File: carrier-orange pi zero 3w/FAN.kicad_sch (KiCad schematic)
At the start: 11 parts, among them J15 FAN1, J16 FAN2, Q3 AO3400A, Q4 AO3400A

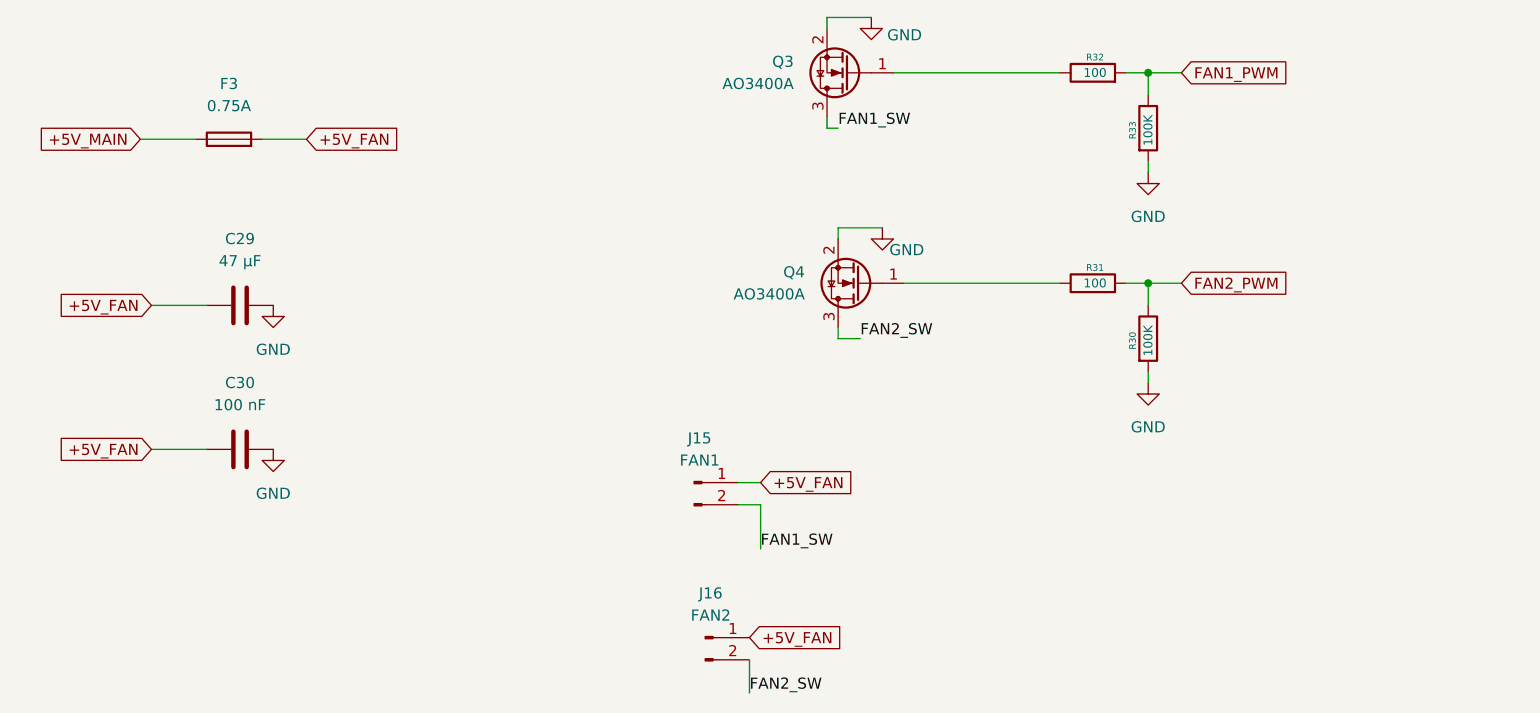
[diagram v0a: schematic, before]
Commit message: ain
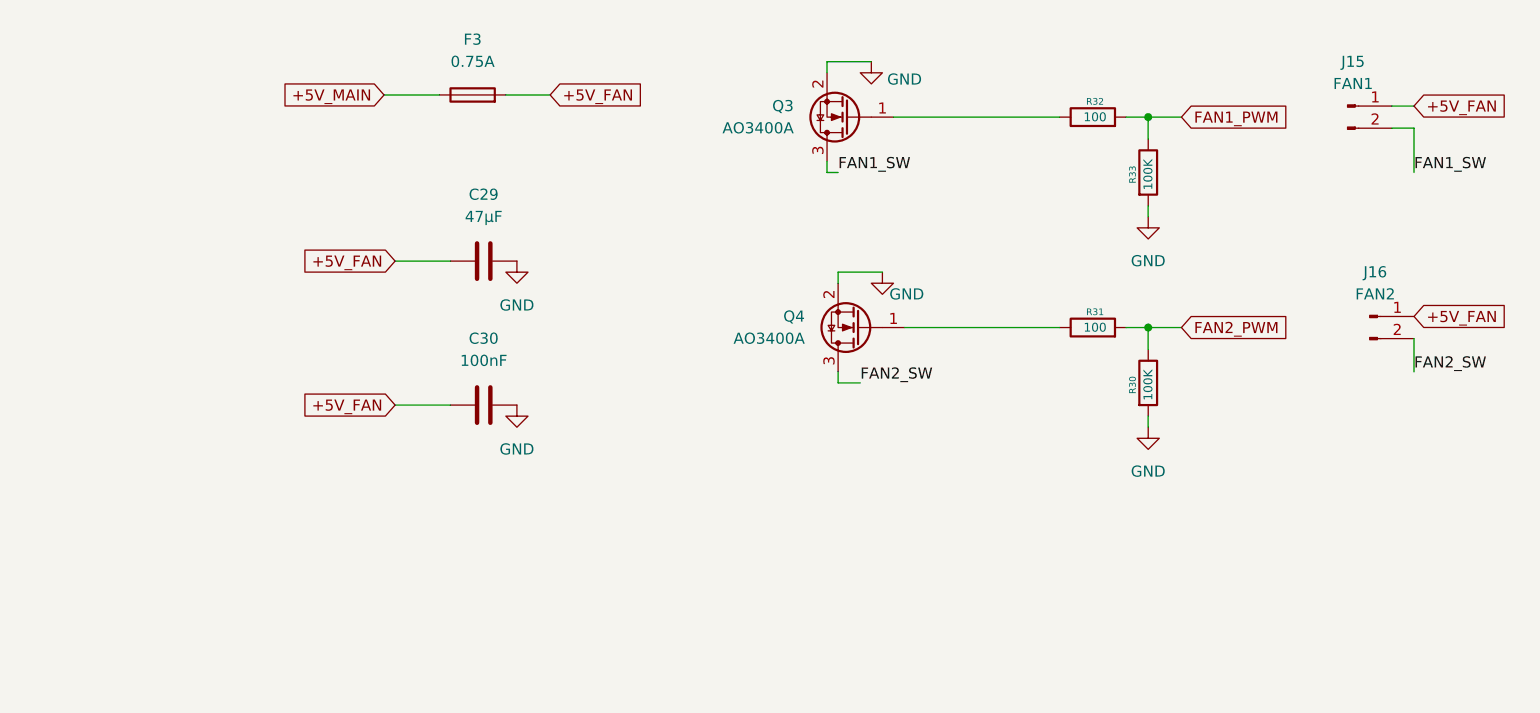
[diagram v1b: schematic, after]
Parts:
- C29: value 47 µF -> 47µF
- C30: value 100 nF -> 100nF
- F3: footprint Capacitor_SMD:C_0805_2012Metric -> Fuse:Fuse_1206_3216Metric
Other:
- moved on the sheet: C29, C30, F3, J15, J16, Q3, Q4, R30, R31, R32, R33

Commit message: ain
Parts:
- J15, J16: footprint Connector_JST:JST_XH_B2B-XH-A_1x02_P2.50mm_Vertical -> Connector_JST:JST_VH_B2P-VH_1x02_P3.96mm_Vertical
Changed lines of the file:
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@@
 			)
 		)
-		(property "Footprint" "Connector_JST:JST_XH_B2B-XH-A_1x02_P2.50mm_Vertical"
+		(property "Footprint" "Connector_JST:JST_VH_B2P-VH_1x02_P3.96mm_Vertical"
 			(at 212.09 44.45 0)
 			(hide yes)
@@
 			)
 		)
-		(property "Footprint" "Connector_JST:JST_XH_B2B-XH-A_1x02_P2.50mm_Vertical"
+		(property "Footprint" "Connector_JST:JST_VH_B2P-VH_1x02_P3.96mm_Vertical"
 			(at 214.63 68.58 0)
 			(hide yes)
